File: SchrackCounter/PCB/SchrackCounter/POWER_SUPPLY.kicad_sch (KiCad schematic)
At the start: 7 parts, among them J1 Conn_01x02_Pin, U1 LM1084-3.3

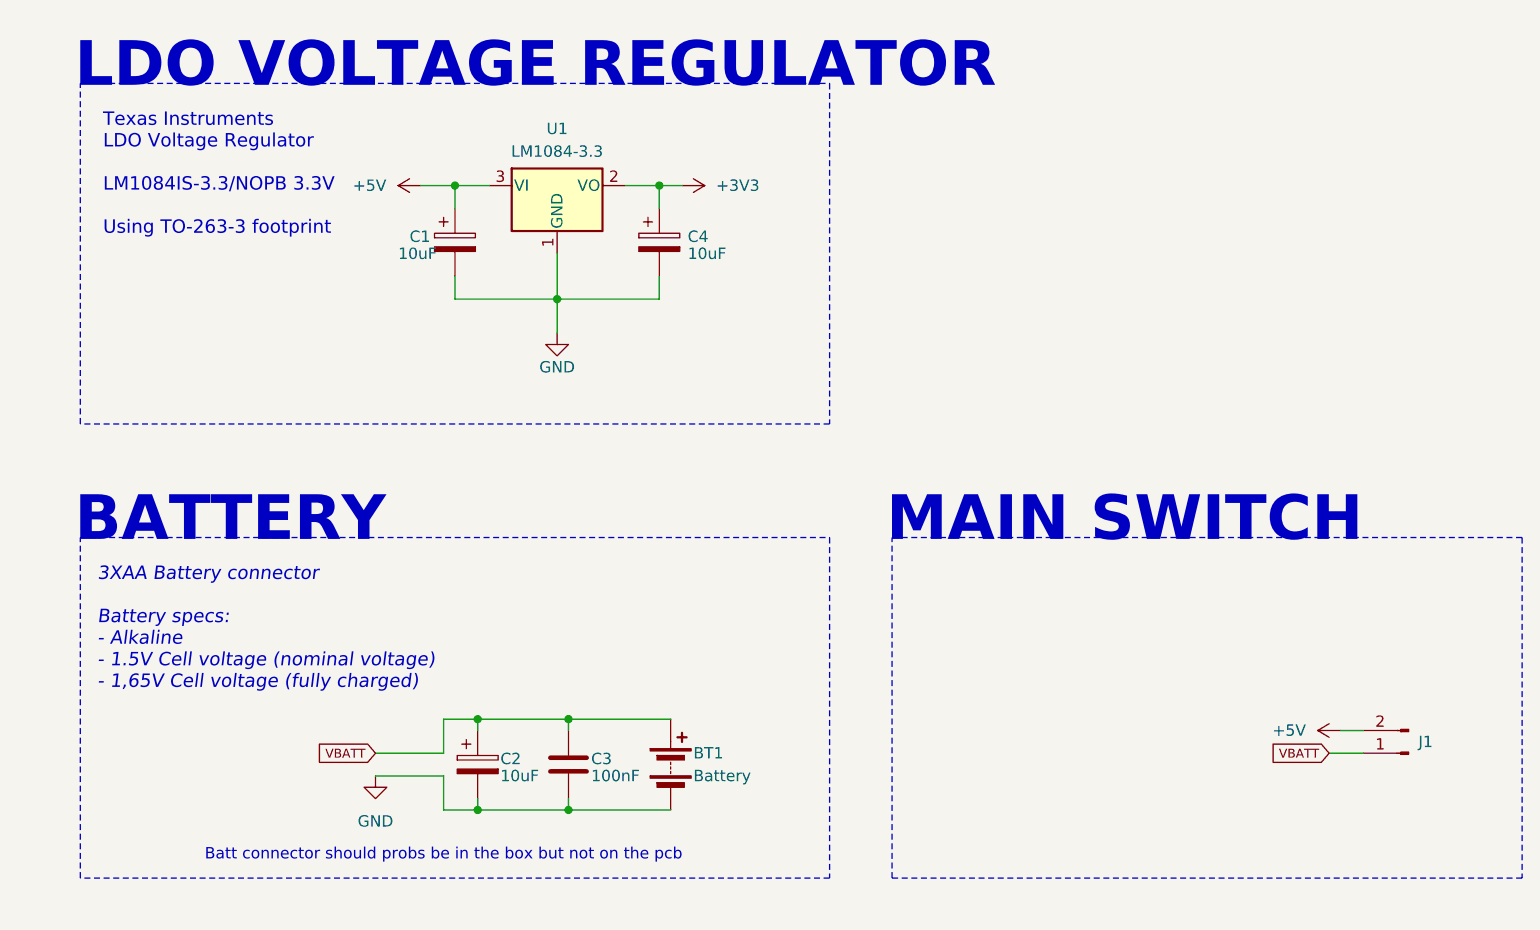
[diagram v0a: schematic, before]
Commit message: PCB update
pcb redesign
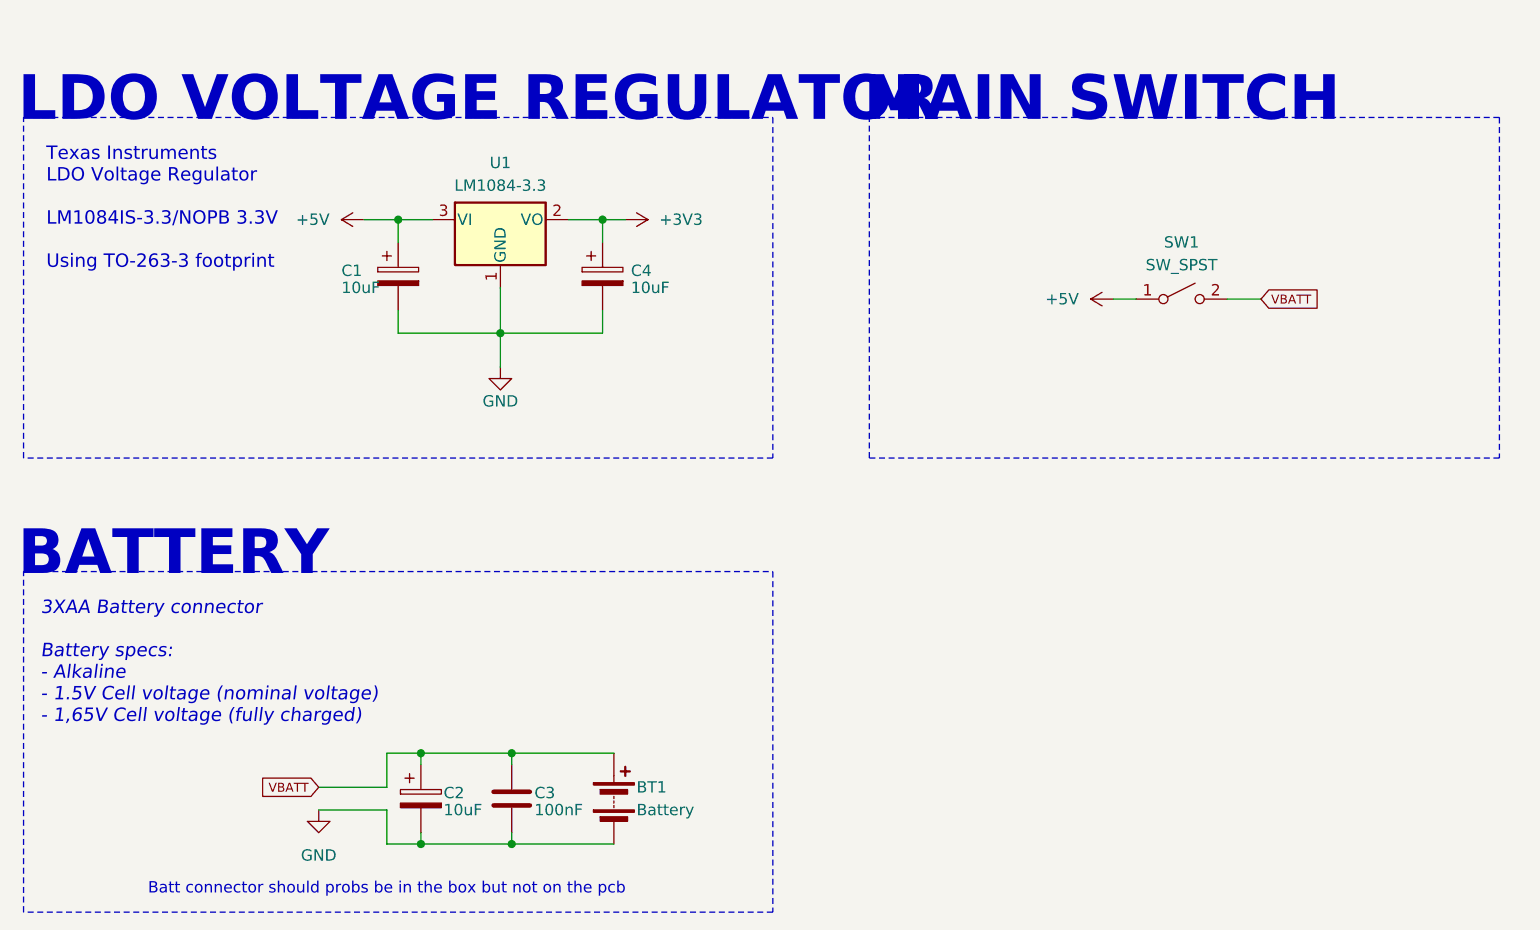
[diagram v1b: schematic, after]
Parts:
- removed J1: Conn_01x02_Pin, Connector_JST:JST_XH_B2B-XH-A_1x02_P2.50mm_Vertical, symbol Connector:Conn_01x02_Pin
- added SW1: SW_SPST, Connector_JST:JST_XH_B2B-XH-A_1x02_P2.50mm_Vertical, symbol Switch:SW_SPST
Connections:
- net +5V: now also SW1.1 (A)
- net VBATT: now also SW1.2 (B)
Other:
- moved on the sheet: BT1, C1, C2, C3, C4, U1
